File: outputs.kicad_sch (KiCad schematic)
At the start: 25 parts, among them J4 Conn_01x02, Q1 SSM3K357R, Q2 SSM3K357R, Q3 SSM3K357R, Q4 SSM3K357R, U10 VNL5050, U11 MCP2551-I-SN, U7 VNL5050, U8 VNL5050, U9 VNL5050

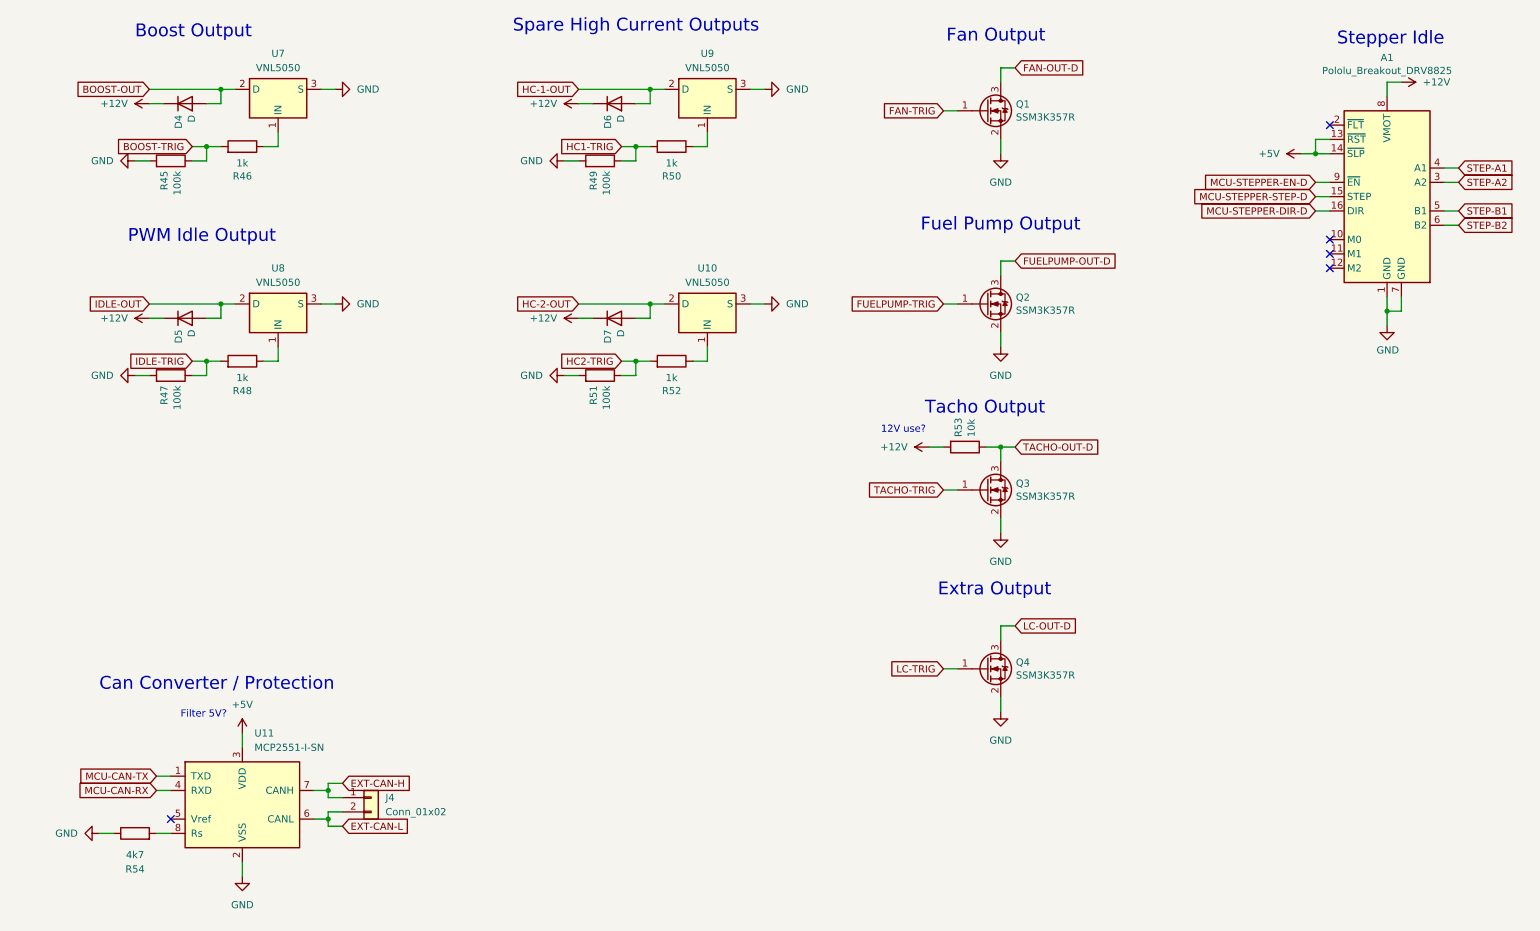
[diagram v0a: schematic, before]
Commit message: Pre MCU switch
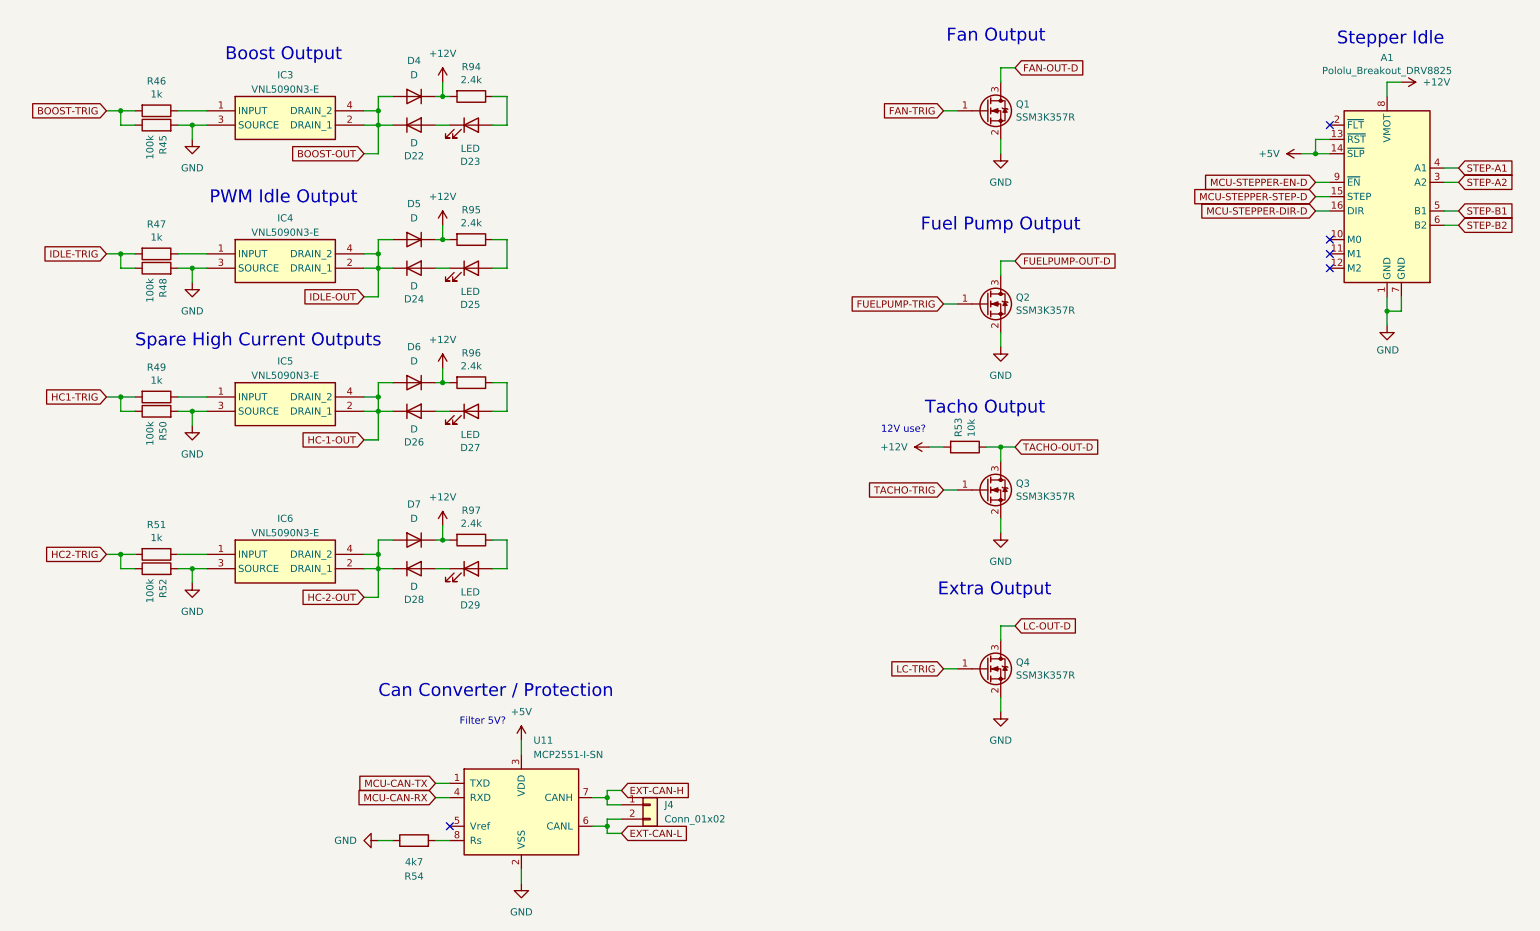
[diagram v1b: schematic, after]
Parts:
- removed U10, U7, U8, U9: VNL5050, IC_Automotive:SOT-223-3_VNL5050, symbol IC_Automotive:VNL5050N3TR
- added D22, D24, D26, D28: D, Diode_SMD:D_SOD-323, symbol Device:D
- added D23, D25, D27, D29: LED, LED_SMD:LED_0805_2012Metric, symbol Device:LED
- added IC3, IC4, IC5, IC6: VNL5090N3-E, SOT230P700X180-4N, symbol IC_Automotive:VNL5090N3-E
- added R94, R95, R96, R97: 2.4k, Resistor_SMD:R_0805_2012Metric, symbol Device:R
- D4, D5, D6, D7: footprint Diode_SMD:D_SOD-123F -> Diode_SMD:D_SOD-323; Digikey Part Number S110FACT-ND -> (none); Manufacturer_Name ONSEMI -> (none); Manufacturer_Part_Number S110FA -> (none); URL https://www.digikey.com/en/products/detail/on-semiconductor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 -> (none)
- R47, R49, R51: value 100k -> 1k; Digikey Part Number 311-100KCRCT-ND -> 311-1.00KCRCT-ND; Manufacturer_Part_Number RC0805FR-07100KL -> RC0805FR-071KL; URL https://www.digikey.com/product-detail/en/yageo/RC0805FR-07100KL/311-100KCRCT-ND/730491 -> https://www.digikey.com/product-detail/en/yageo/RC0805FR-071KL/311-1.00KCRCT-ND/730391
- R48, R50, R52: value 1k -> 100k; Digikey Part Number 311-1.00KCRCT-ND -> 311-100KCRCT-ND; Manufacturer_Part_Number RC0805FR-071KL -> RC0805FR-07100KL; URL https://www.digikey.com/product-detail/en/yageo/RC0805FR-071KL/311-1.00KCRCT-ND/730391 -> https://www.digikey.com/product-detail/en/yageo/RC0805FR-07100KL/311-100KCRCT-ND/730491
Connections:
- net +12V: now also R94.2, R95.2, R96.2, R97.2
- net BOOST-OUT: now also D22.1 (K), IC3.2 (DRAIN_1), IC3.4 (DRAIN_2)
- net GND: now also R48.2, R50.2, R52.2, IC3.3 (SOURCE), IC4.3 (SOURCE), IC5.3 (SOURCE), IC6.3 (SOURCE); no longer R47.2, R49.2, R51.2
- net HC-1-OUT: now also D26.1 (K), IC5.2 (DRAIN_1), IC5.4 (DRAIN_2)
- net HC-2-OUT: now also D28.1 (K), IC6.2 (DRAIN_1), IC6.4 (DRAIN_2)
- net HC1-TRIG: now also R49.2, R50.1; no longer R49.1, R50.2
- net HC2-TRIG: now also R51.2, R52.1; no longer R51.1, R52.2
- net IDLE-OUT: now also D24.1 (K), IC4.2 (DRAIN_1), IC4.4 (DRAIN_2)
- net IDLE-TRIG: now also R47.2, R48.1; no longer R47.1, R48.2
- net at R46.1: now also IC3.1 (INPUT)
- new net: D24.2 (A), D25.1 (K)
- new net: D26.2 (A), D27.1 (K)
- new net: D27.2 (A), R96.1
- new net: D25.2 (A), R95.1
- new net: D23.2 (A), R94.1
- new net: IC4.1 (INPUT), R47.1
- new net: D29.2 (A), R97.1
- new net: D28.2 (A), D29.1 (K)
- new net: D22.2 (A), D23.1 (K)
- new net: IC6.1 (INPUT), R51.1
- new net: IC5.1 (INPUT), R49.1
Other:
- moved on the sheet: J4, R45, R46, R54, U11
